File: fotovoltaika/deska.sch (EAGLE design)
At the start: 19 parts

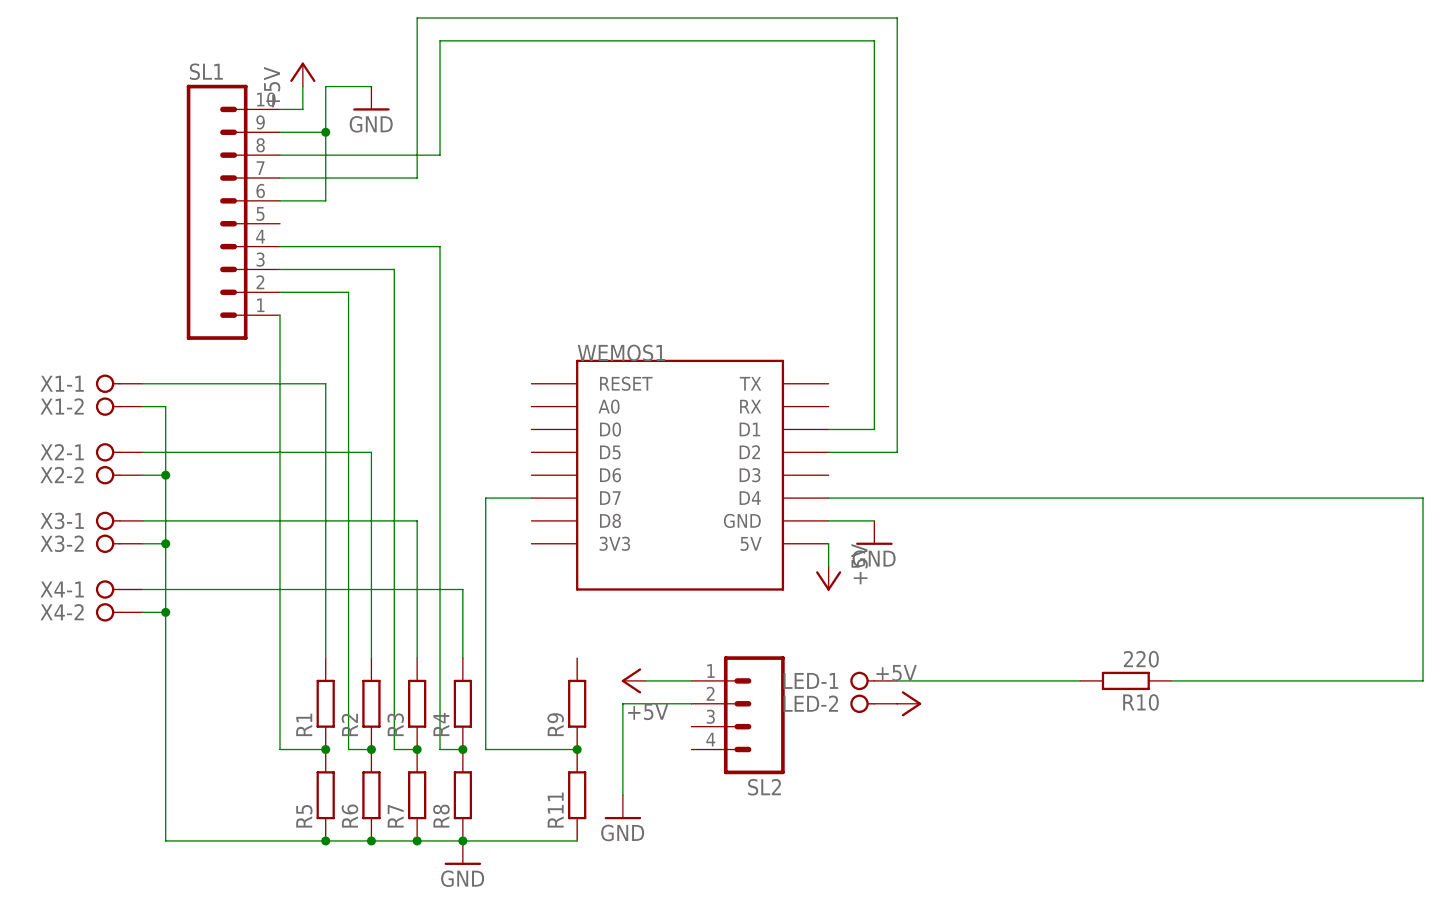
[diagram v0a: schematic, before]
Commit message: upravy desek
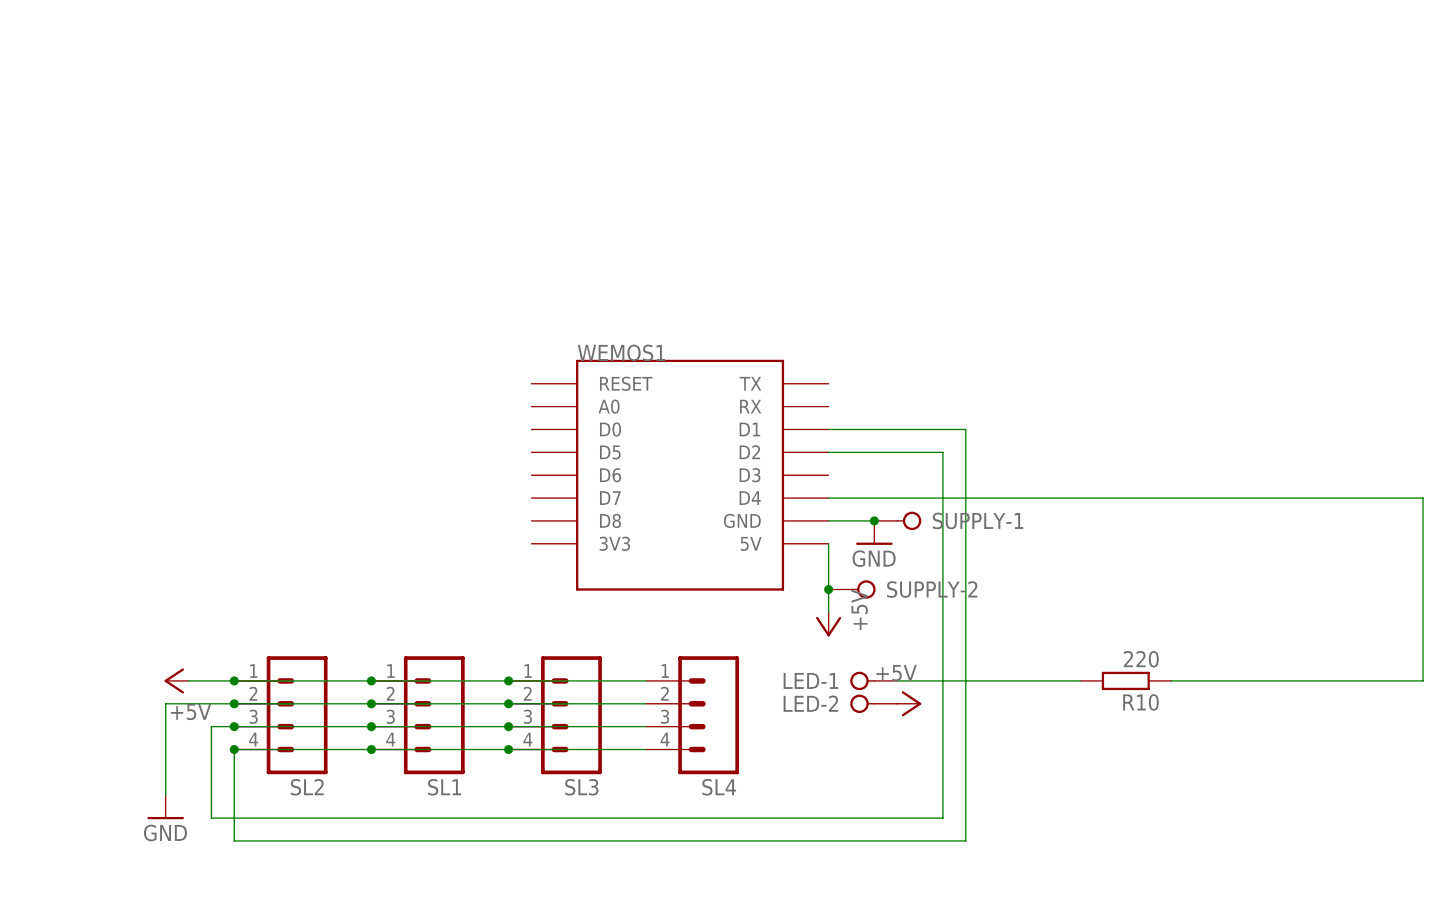
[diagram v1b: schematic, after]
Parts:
- removed R1, R11, R2, R3, R4, R5, R6, R7, R8, R9: (no value), rcl:R-EU_0207/7
- removed X1, X2, X3, X4: (no value), con-wago-508:W237-02P
- added SL3, SL4: (no value), con-amp-quick:M04
- added SUPPLY: (no value), con-wago-508:W237-02P
- SL1: device con-amp-quick:M10 -> con-amp-quick:M04
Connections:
- removed net N$10: R4.2, X4-1.KL
- removed net N$13: R11.2, R9.1, WEMOS1.D7
- removed net N$3: R1.2, X1-1.KL
- removed net N$4: R1.1, R5.2, SL1.1
- removed net N$5: R2.1, R6.2, SL1.2
- removed net N$6: R3.1, R7.2, SL1.3
- removed net N$7: R4.1, R8.2, SL1.4
- removed net N$8: R2.2, X2-1.KL
- removed net N$9: R3.2, X3-1.KL
- net +5V: now also SL1.1, SL3.1, SL4.1, SUPPLY-2.KL; no longer SL1.10
- net GND: now also SL1.2, SL3.2, SL4.2, SUPPLY-1.KL; no longer R11.1, R5.1, R6.1, R7.1, R8.1, SL1.6, SL1.9, X1-2.KL, X2-2.KL, X3-2.KL, X4-2.KL
- net N$1: now also SL1.4, SL2.4, SL3.4, SL4.4, WEMOS1.D1; no longer SL1.7, WEMOS1.D2
- net N$2: now also SL1.3, SL2.3, SL3.3, SL4.3, WEMOS1.D2; no longer SL1.8, WEMOS1.D1
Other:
- moved on the sheet: SL2
